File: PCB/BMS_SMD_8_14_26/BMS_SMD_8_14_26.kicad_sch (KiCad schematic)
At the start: 22 parts, among them J1 ADS_1115, J2 MP_OUT-, J3 MP_OUT+, J4 MP_VIN-, J5 MP_VIN+, J6 VTAP_INPUTS, J7 MCU_PINS, U1 INA180A1, U2 ESP32-S3-WROOM-1

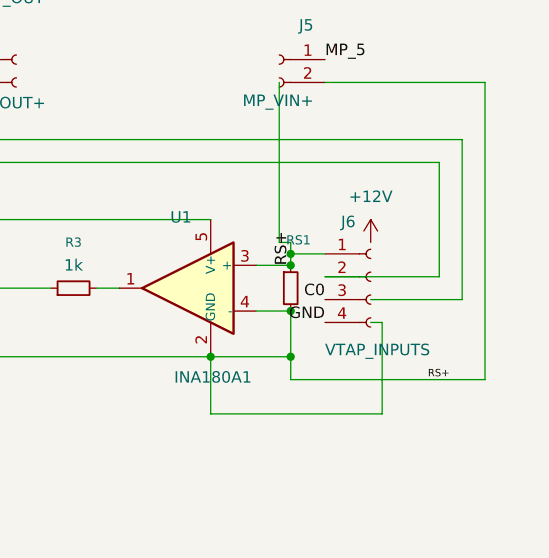
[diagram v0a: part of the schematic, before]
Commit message: WIP: recover pre-repair project reorganization
Restores reorganized source, tests, GUI harnesses, and current development files. Eleven unit tests pass; measurement-report and integration tests remain work in progress.
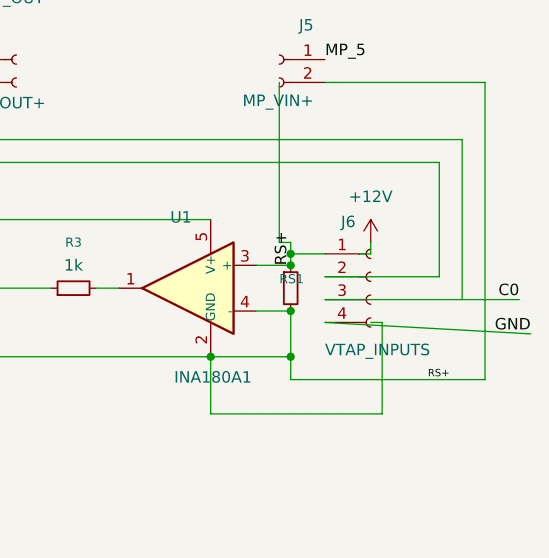
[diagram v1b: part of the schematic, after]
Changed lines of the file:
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@@
+	(wire
+		(pts
+			(xy 191.77 105.41) (xy 191.77 106.68)
+		)
+		(stroke
+			(width 0)
+			(type default)
+		)
+	)
 	(wire
 		(pts
@@
 	(wire
 		(pts
-			(xy 191.77 111.76) (xy 201.93 111.76)
-		)
-		(stroke
-			(width 0)
-			(type default)
-		)
-	)
-	(wire
-		(pts
 			(xy 132.08 134.62) (xy 132.08 124.46)
 		)
@@
 	(wire
 		(pts
+			(xy 190.5 106.68) (xy 191.77 106.68)
+		)
+		(stroke
+			(width 0)
+			(type default)
+		)
+	)
+	(wire
+		(pts
+			(xy 209.55 115.57) (xy 186.69 114.3)
+		)
+		(stroke
+			(width 0)
+			(type default)
+		)
+	)
+	(wire
+		(pts
 			(xy 193.04 124.46) (xy 173.99 124.46)
 		)
@@
 		(pts
 			(xy 100.33 60.96) (xy 125.73 60.96)
+		)
+		(stroke
+			(width 0)
+			(type default)
+		)
+	)
+	(wire
+		(pts
+			(xy 186.69 111.76) (xy 208.28 111.76)
 		)
 		(stroke
@@
 	)
 	(label "GND"
-		(at 186.69 114.3 180)
+		(at 209.55 115.57 180)
 		(effects
 			(font
@@
 	)
 	(label "C0"
-		(at 186.69 111.76 180)
+		(at 208.28 111.76 180)
 		(effects
 			(font
@@
 		(dnp no)
 		(property "Reference" "RS1"
-			(at 182.372 105.156 0)
-			(show_name no)
-			(do_not_autoplace no)
+			(at 181.61 109.474 0)
+			(show_name no)
+			(do_not_autoplace no)
